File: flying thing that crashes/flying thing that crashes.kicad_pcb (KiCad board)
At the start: 2 copper layers, 83 parts, among them J1 RMotor, J2 LMotor, J3 J3, J4 J4, M1 Motor_Servo, M2 Motor_Servo, M3 Motor_Servo, M4 Motor_Servo, M5 Motor_Servo, M6 Motor_Servo, M7 Motor_Servo, M8 Motor_Servo, U1 PCA9685PW, U2 Ai-Thinker-Ra-02, U3 Ai-Thinker-Ra-02, U4 AMS1117-3.3, U5 MPU-9250, U6 TPS63070RNMR

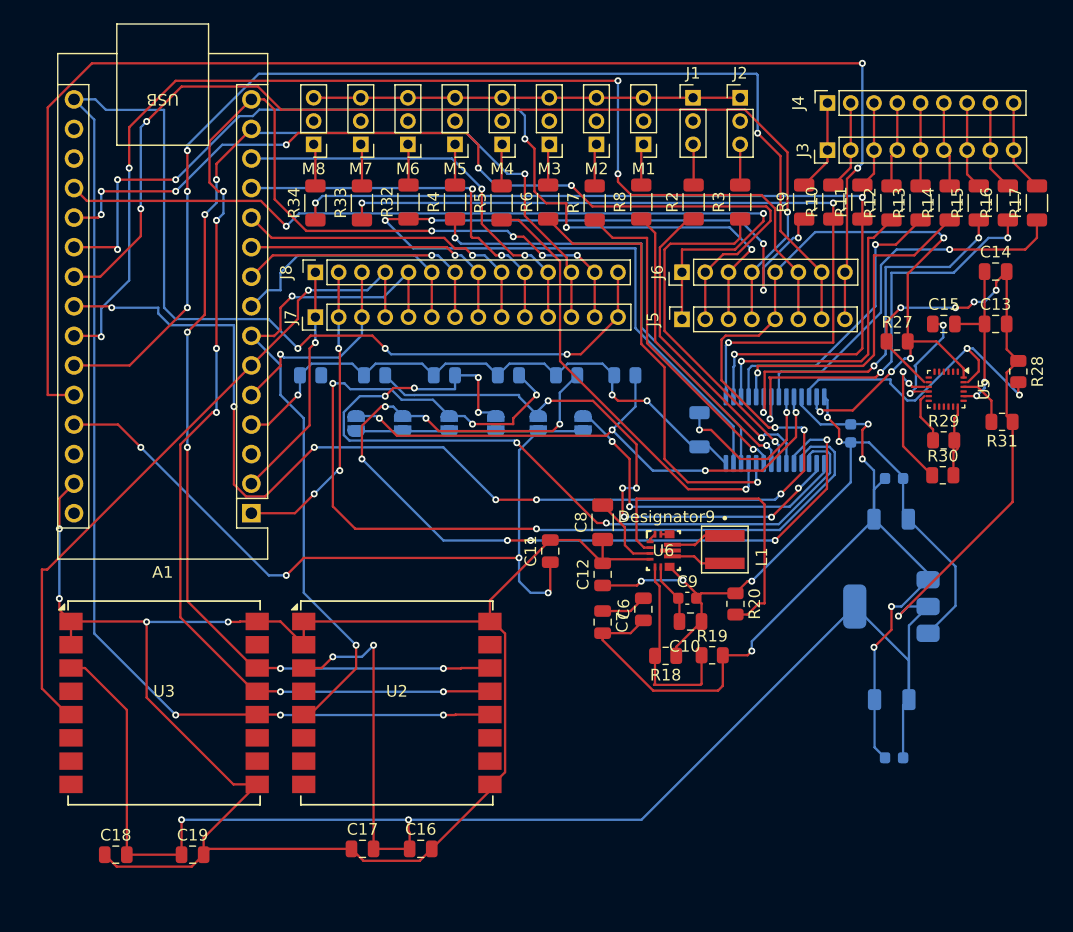
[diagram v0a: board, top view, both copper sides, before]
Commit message: controller
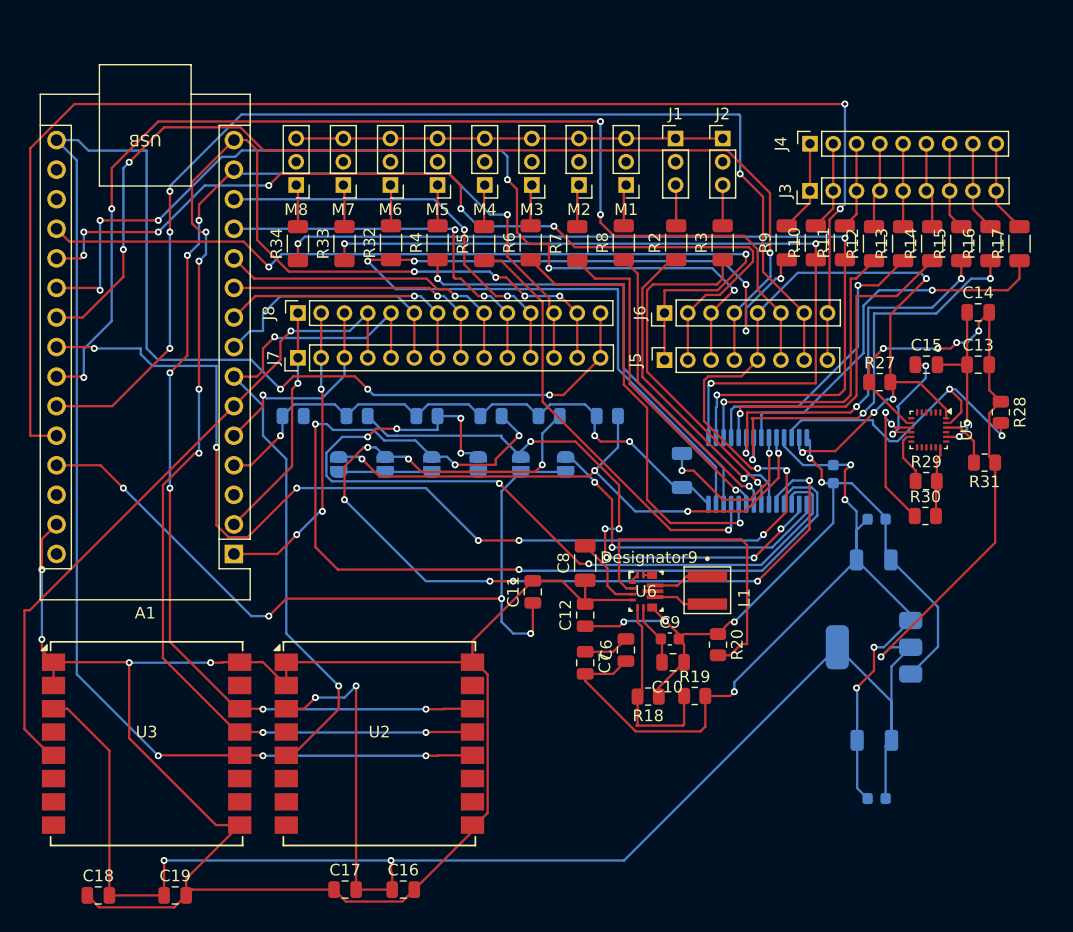
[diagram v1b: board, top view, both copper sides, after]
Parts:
- moved C6 3.81 mm to (65.7, 64.9)
- moved A1 3.81 mm to (32.0, 56.7)
- moved C1 3.81 mm to (83.5, 49.8)
- moved C10 3.81 mm to (69.7, 66.0)
- moved C11 3.81 mm to (57.7, 59.9)
- moved C12 3.81 mm to (62.2, 61.9)
- moved C13 3.81 mm to (96.0, 40.4)
- moved C14 3.81 mm to (96.0, 35.9)
- moved C15 3.81 mm to (91.5, 40.4)
- moved C16 3.81 mm to (46.5, 85.5)
- moved C17 3.81 mm to (41.5, 85.5)
- moved C18 3.81 mm to (20.4, 86.0)
- moved C19 3.81 mm to (26.9, 86.0)
- moved C2 3.81 mm to (87.2, 53.7)
- moved C3 3.81 mm to (87.0, 57.2)
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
